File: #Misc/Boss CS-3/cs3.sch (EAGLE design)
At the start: 105 parts, among them IC1 IC99, IC2 IC2, IC4 uPC4558C, IC5 HA1457, Q1 2SC732TM-GR, Q2 2SC945-P, Q3 2SC945-P, Q4 2SK30A, Q5 2SK30A, SW1 MOMENTARY

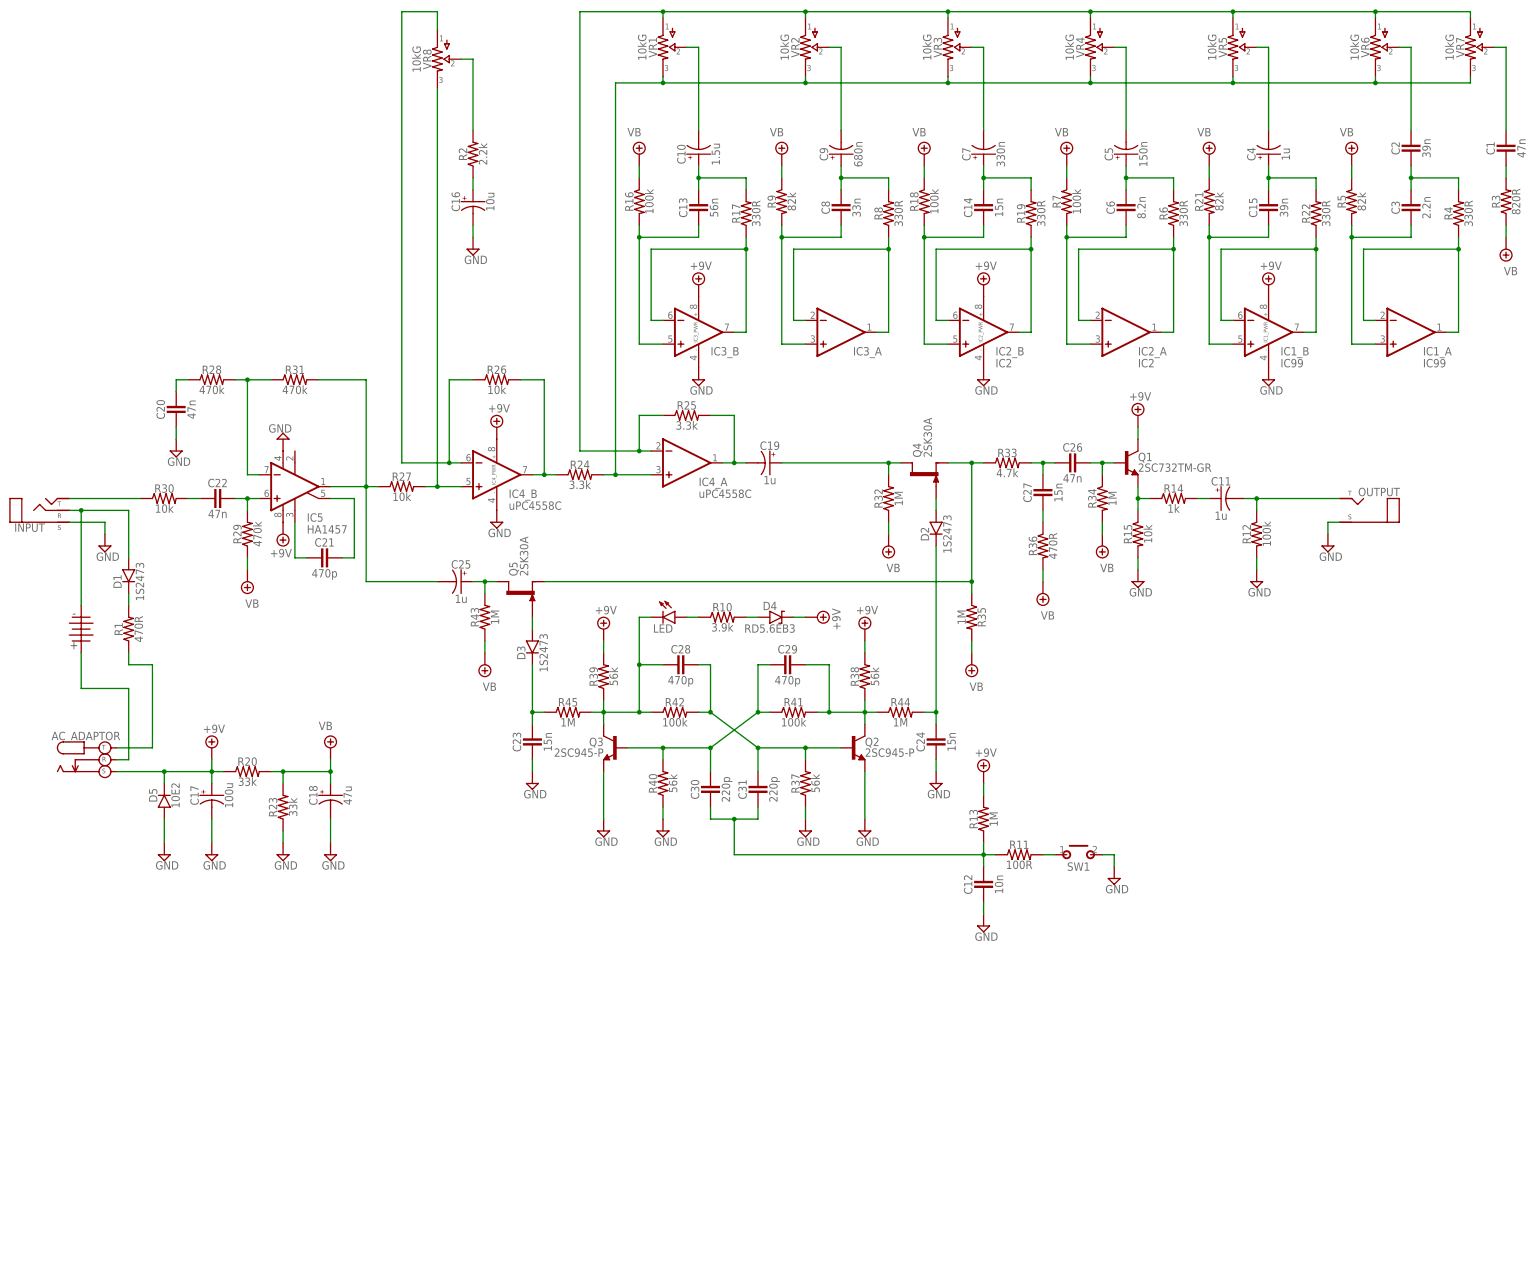
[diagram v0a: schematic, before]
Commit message: 20180207
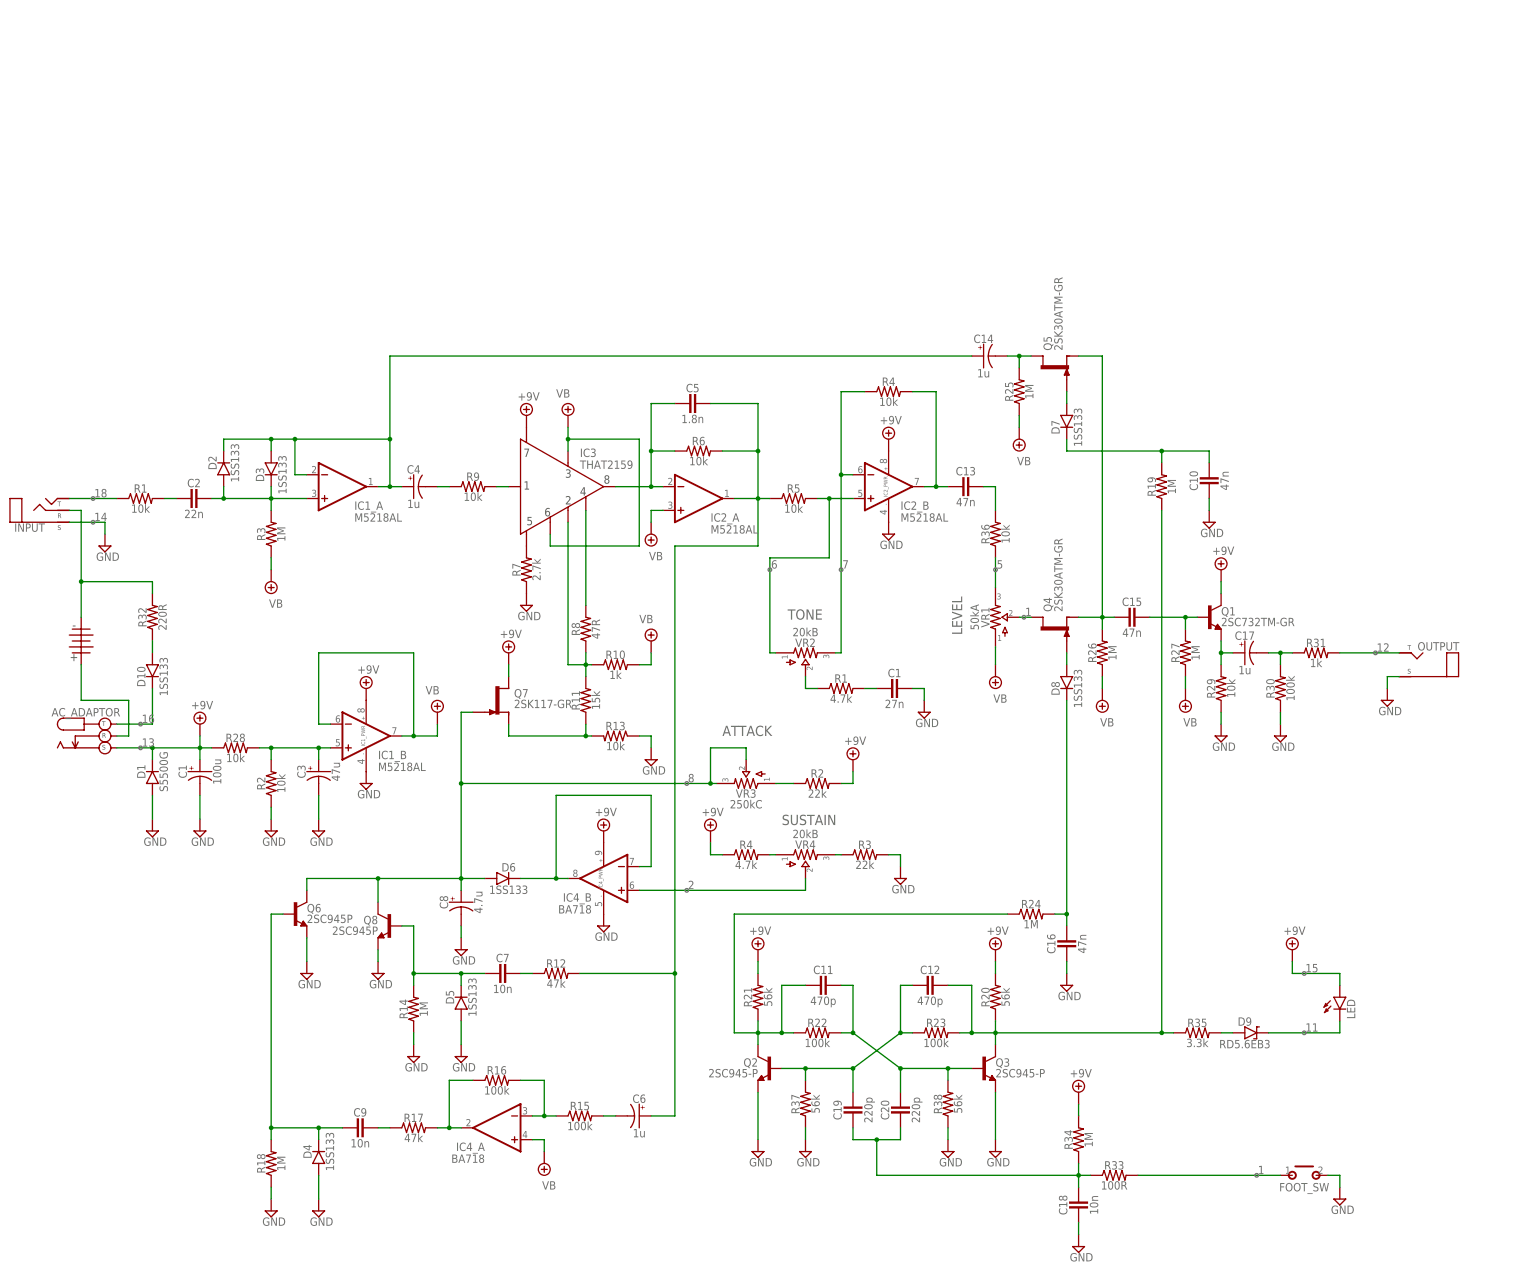
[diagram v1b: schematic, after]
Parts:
- removed BATTERY: BATTERY, pedals-jacks:BATTERY
- removed C21, C28, C29: 470p, pedals-capacitors-film:CER/FILMBOX.1
- removed C22, C26: 47n, pedals-capacitors-film:CER/FILMBOX.1
- removed C23, C24, C27: 15n, pedals-capacitors-film:CER/FILMBOX.1
- removed C25: 1u, pedals-capacitors-elec:0400
- removed C30, C31: 220p, pedals-capacitors-film:CER/FILMBOX.1
- removed IC5: HA1457, pedals-integrated circuits:HA1457
- removed R39, R40: 56k, pedals-resistors:R_.3B
- removed R41, R42: 100k, pedals-resistors:R_.3B
- removed R43, R44, R45: 1M, pedals-resistors:R_.3B
- removed SW1: MOMENTARY, pedals-switches:MOMENTARY
- removed VR5, VR6, VR7, VR8: 10kG, pedals-potentiometers:POTS16MM
- added 1101: BATTERY, pedals-jacks:BATTERY
- added C1 : 27n, pedals-capacitors-film:CER/FILMBOX.1
- added D10, D6, D7, D8: 1SS133, pedals-diodes:DO35.2
- added D9: RD5.6EB3, pedals-diodes:ZENER.2
- added FOOT_SW: MOMENTARY, pedals-switches:MOMENTARY
- added Q6, Q8: 2SC945P, pedals-transistors:2N3904
- added Q7: 2SK117-GR, pedals-transistors:2N5457
- added R1 : 4.7k, pedals-resistors:R_.3B
- added R2 : 22k, pedals-resistors:R_.3B
- added R3 : 22k, pedals-resistors:R_.3B
- added R4 : 4.7k, pedals-resistors:R_.3B
- C1: value 47n -> 100u; device pedals-capacitors-film:CER/FILMBOX.1 -> pedals-capacitors-elec:0400
- C10: value 1.5u -> 47n; device pedals-capacitors-elec:0400 -> pedals-capacitors-film:CER/FILMBOX.1
- C11: value 1u -> 470p; device pedals-capacitors-elec:0400 -> pedals-capacitors-film:CER/FILMBOX.1
- C12: value 10n -> 470p
- C13: value 56n -> 47n
- C14: value 15n -> 1u; device pedals-capacitors-film:CER/FILMBOX.1 -> pedals-capacitors-elec:0400
- C15: value 39n -> 47n
- C16: value 10u -> 47n; device pedals-capacitors-elec:0400 -> pedals-capacitors-film:CER/FILMBOX.1
- C17: value 100u -> 1u
- C18: value 47u -> 10n; device pedals-capacitors-elec:0400 -> pedals-capacitors-film:CER/FILMBOX.1
- C19: value 1u -> 220p; device pedals-capacitors-elec:0400 -> pedals-capacitors-film:CER/FILMBOX.1
- C2: value 39n -> 22n
- C20: value 47n -> 220p
- C3: value 2.2n -> 47u; device pedals-capacitors-film:CER/FILMBOX.1 -> pedals-capacitors-elec:0400
- C5: value 150n -> 1.8n; device pedals-capacitors-elec:0400 -> pedals-capacitors-film:CER/FILMBOX.1
- C6: value 8.2n -> 1u; device pedals-capacitors-film:CER/FILMBOX.1 -> pedals-capacitors-elec:0400
- C7: value 330n -> 10n; device pedals-capacitors-elec:0400 -> pedals-capacitors-film:CER/FILMBOX.1
- C8: value 33n -> 4.7u; device pedals-capacitors-film:CER/FILMBOX.1 -> pedals-capacitors-elec:0400
- C9: value 680n -> 10n; device pedals-capacitors-elec:0400 -> pedals-capacitors-film:CER/FILMBOX.1
- D1: value 1S2473 -> S5500G
- D2, D3: value 1S2473 -> 1SS133
- D4: value RD5.6EB3 -> 1SS133; device pedals-diodes:ZENER.2 -> pedals-diodes:DO35.2
- D5: value 10E2 -> 1SS133
- IC1: value IC99 -> M5218AL
- IC2: value IC2 -> M5218AL
- IC3: value (none) -> THAT2159; device pedals-integrated circuits:DUALTH -> pedals-integrated circuits:THAT2181C
- IC4: value uPC4558C -> BA718; device pedals-integrated circuits:DUALTH -> pedals-integrated circuits:DUAL
- Q1: device pedals-transistors:2SC828A -> pedals-transistors:2N3904
- Q4, Q5: value 2SK30A -> 2SK30ATM-GR
- R1, R36: value 470R -> 10k
- R10: value 3.9k -> 1k
- R11: value 100R -> 15k
- R12: value 100k -> 47k
- R13: value 1M -> 10k
- R14: value 1k -> 1M
- R15, R30: value 10k -> 100k
- R17: value 330R -> 47k
- R18: value 100k -> 1M
- R19: value 330R -> 1M
- R2: value 2.2k -> 10k
- R20: value 33k -> 56k
- R21: value 82k -> 56k
- R22: value 330R -> 100k
- R23: value 33k -> 100k
- R24, R25: value 3.3k -> 1M
- R26, R27: value 10k -> 1M
- R28, R29: value 470k -> 10k
- R3: value 820R -> 1M
- R31: value 470k -> 1k
- R32: value 1M -> 220R
- R33: value 4.7k -> 100R
- R35: value 1M -> 3.3k
- R4, R6: value 330R -> 10k
- R5, R9: value 82k -> 10k
- R7: value 100k -> 2.7k
- R8: value 330R -> 47R
- VR1: value 10kG -> 50kA
- VR2, VR4: value 10kG -> 20kB
- VR3: value 10kG -> 250kC
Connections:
- removed net N$56: IC1_A.-IN, IC1_A.OUT, R4.1
- removed net N$57: C3.2, IC1_A.+IN, R5.2
- removed net N$58: C2.2, C3.1, R4.2
- removed net N$59: C2.1, VR6.2
- removed net N$60: C1.2, R3.2
- removed net N$61: C1.1, VR7.2
- removed net N$62: C11.-, OUTPUT.TIP, R12.1
- removed net N$63: C23.1, D3.C, R45.1
- removed net N$64: C24.1, D2.C, R44.2
- removed net N$65: R11.2, SW1.P
- removed net N$66: LED.A, R10.1
- removed net N$67: D4.A, R10.2
- new net N$75: C12.1, Q3.C, R19.1, R20.1, R23.2, R35.1
- net +9V: now also C1.+, D1.C, IC3.P$7, LED.A, Q7.D, R20.2, R21.2, R28.1, R2 .2, R34.2, R4 .1; no longer C17.+, D4.C, D5.C, IC3_PWR.V+, IC5.V+, R13.2, R20.1, R38.2, R39.2
- net GND: now also C1.-, C10.2, C16.2, C18.2, C1 .2, C3.-, C8.-, D1.A, D4.A, FOOT_SW.S, Q6.E, Q8.E, R13.1, R14.1, R18.1, R2.1, R29.1, R30.1, R38.1, R3 .2, R7.1; no longer C12.2, C16.-, C17.-, C18.-, C20.2, C23.2, C24.2, IC3_PWR.V-, IC5.V-, R12.2, R15.2, R23.1, R40.1, SW1.S
- net N$1: now also C3.+, IC1_B.+IN, R2.2, R28.2; no longer C21.2, IC5.ON1
- net N$10: now also C4.-, R9.1; no longer IC4_B.-IN, R26.1, VR8.1
- net N$11: now also IC3.P$1, R9.2; no longer IC4_B.OUT, R24.1, R26.2
- net N$12: now also IC3.P$4, R8.2; no longer IC4_B.+IN, R27.2, VR8.3
- net N$13: now also IC3.P$2, R10.1, R11.2, R8.1; no longer IC4_A.+IN, R24.2, VR1.3, VR2.3, VR3.3, VR4.3, VR5.3, VR6.3, VR7.3
- net N$14: now also Q7.S, R11.1, R13.2; no longer IC4_A.-IN, R25.1, VR1.1, VR2.1, VR3.1, VR4.1, VR5.1, VR6.1, VR7.1
- net N$15: now also C5.2, IC2_A.-IN, IC3.P$8, R6.1; no longer C19.-, IC4_A.OUT, R25.2
- net N$16: now also C17.+, Q1.E, R29.2; no longer R2.2, VR8.2
- net N$17: now also IC2_B.+IN, R5.2, VR2.1; no longer C16.+, R2.1
- net N$18: now also IC2_B.-IN, R4.1, VR2.3; no longer IC3_B.-IN, IC3_B.OUT, R17.1
- net N$19: now also IC2_B.OUT, R4.2; no longer IC3_B.+IN, R16.2
- net N$2: now also INPUT.T, R1.1; no longer BATTERY.P$2, D1.A, INPUT.R
- net N$20: now also R36.2; no longer C10.+, R17.2
- net N$21: now also R36.1, VR1.3; no longer C10.-, VR1.2
- net N$22: now also R1 .1, VR2.2; no longer C19.+, Q4.D, R32.2
- net N$23: now also C1 .1, R1 .2; no longer C25.+, Q5.D, R43.2
- net N$24: now also C14.-, Q5.D, R25.2; no longer IC3_A.-IN, IC3_A.OUT, R8.1
- net N$25: now also Q4.D, VR1.2; no longer C8.2, IC3_A.+IN, R9.2
- net N$26: now also C15.2, Q4.S, Q5.S, R26.2; no longer C8.1, C9.+, R8.2
- net N$27: now also 1101.P$1; no longer BATTERY.P$1
- net N$28: now also 1101.P$2, INPUT.R, R32.2; no longer AC_ADAPTOR.T, R1.1
- net N$29: now also C11.2, Q2.C, R21.1, R22.1, R24.1; no longer C28.2, LED.C, Q3.C, R39.1, R42.1, R45.2
- net N$3: now also AC_ADAPTOR.T, D10.C; no longer C21.1, IC5.ON2
- net N$30: now also C15.1, Q1.B, R27.2; no longer D1.C, R1.2
- net N$31: now also D8.A, Q4.G; no longer C29.1, Q2.C, R38.1, R41.2, R44.1
- net N$32: now also C12.2, C19.1, Q2.B, R23.1, R37.2; no longer C29.2, C30.1, Q3.B, R40.2, R41.1
- net N$33: now also D7.A, Q5.G; no longer C9.-, VR2.2
- net N$34: now also C11.1, C20.1, Q3.B, R22.2, R38.2; no longer C28.1, C31.1, Q2.B, R37.2, R42.2
- net N$35: now also IC4_B.+IN, VR4.2; no longer D3.A, Q5.G
- net N$36: now also R2 .1, VR3.1; no longer C12.1, C30.2, C31.2, R11.1, R13.1
- net N$37: now also C8.+, D6.A, Q6.C, Q7.G, Q8.C, VR3.2, VR3.3; no longer D2.A, Q4.G
- net N$38: now also D6.C, IC4_B.-IN, IC4_B.OUT; no longer IC2_B.-IN, IC2_B.OUT, R19.1
- net N$39: now also R4 .2, VR4.1; no longer C14.2, IC2_B.+IN, R18.2
- net N$4: now also D10.A, R32.1; no longer INPUT.T, R30.1
- net N$40: now also R3 .1, VR4.3; no longer C14.1, C7.+, R19.2
- net N$41: now also C9.2, D4.C, Q6.B, R18.2; no longer C7.-, VR3.2
- net N$42: now also C7.2, D5.C, Q8.B, R14.2; no longer Q4.S, Q5.S, R33.1, R35.1
- net N$43: now also C7.1, R12.1; no longer C26.2, C27.1, R33.2
- net N$44: now also C9.1, R17.1; no longer IC2_A.-IN, IC2_A.OUT, R6.1
- net N$45: now also IC4_A.OUT, R16.1, R17.2; no longer C6.2, IC2_A.+IN, R7.2
- net N$46: now also C17.-, R30.2, R31.1; no longer C5.+, C6.1, R6.2
- net N$47: now also IC4_A.-IN, R15.1, R16.2; no longer C5.-, VR4.2
- net N$48: now also C6.-, R15.2; no longer C27.2, R36.1
- net N$49: now also OUTPUT.TIP, R31.2; no longer C26.1, Q1.B, R34.1
- net N$5: now also C2.2, R1.2; no longer C22.2, R30.2
- net N$50: now also C5.1, C6.+, IC2_A.OUT, R12.2, R5.1, R6.2; no longer IC1_B.-IN, IC1_B.OUT, R22.1
- net N$51: now also C10.1, D7.C, R19.2; no longer C15.2, IC1_B.+IN, R21.2
- net N$52: now also C16.1, D8.C, R24.2; no longer C15.1, C4.+, R22.2
- net N$53: now also D9.A, R35.2; no longer C4.-, VR5.2
- net N$54: now also D9.C, LED.C; no longer Q1.E, R14.1, R15.1
- net N$55: now also FOOT_SW.P, R33.2; no longer C11.+, R14.2
- net N$6: now also C18.1, C19.2, C20.2, R33.1, R34.1; no longer C22.1, IC5.+IN, R29.2
- net N$7: now also C2.1, D2.A, D3.C, IC1_A.+IN, R3.2; no longer IC5.-IN, R28.2, R31.1
- net N$8: now also C14.+, C4.+, D2.C, D3.A, IC1_A.-IN, IC1_A.OUT; no longer C25.-, IC5.OUT, R27.1, R31.2
- net N$9: now also IC3.P$5, R7.2; no longer C20.1, R28.1
- net VB: now also IC1_B.-IN, IC1_B.OUT, IC2_A.+IN, IC3.P$3, IC3.P$6, IC4_A.+IN, R10.2, R25.1, R26.1, R27.1, VR1.1; no longer C18.+, R16.1, R18.1, R20.2, R21.1, R23.2, R29.1, R32.1, R34.2, R35.2, R36.2, R43.1, R5.1, R7.1, R9.1
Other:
- note added: "1"
- note added: "11"
- note added: "12"
- note added: "13"
- note added: "14"
- note added: "15"
- note added: "16"
- note added: "18"
- note added: "2"
- note added: "5"
- note added: "6"
- note added: "7"
- note added: "8"
- note added: "ATTACK"
- note added: "LEVEL"
- note added: "SUSTAIN"
- note added: "TONE"
- moved on the sheet: AC_ADAPTOR, C12, C13, C15, C17, C2, C20, C4, D1, D2, D3, D5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
